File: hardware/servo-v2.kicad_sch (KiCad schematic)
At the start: 44 parts

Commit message: fix symbols
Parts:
- C1, C12: value (none) -> 10uF; footprint (none) -> kicad-libraries:C0805
- C10, C11: value (none) -> 100nF; footprint (none) -> kicad-libraries:C0603
- C2: value (none) -> 1uF; footprint (none) -> kicad-libraries:C0603F
- C3, C4, C5: value (none) -> 100nF; footprint (none) -> kicad-libraries:C0603F
- C6: value (none) -> 220nF; footprint (none) -> kicad-libraries:C0603F
- C7: value (none) -> 220pF; footprint (none) -> kicad-libraries:C0402F
- C8, C9: value (none) -> 10pF; footprint (none) -> kicad-libraries:C0603F
- D1: value (none) -> Z12V; footprint (none) -> kicad-libraries:SOD-123
- D3: value (none) -> blue; footprint (none) -> kicad-libraries:D0603E
- P1: value (none) -> CON-SENSOR2; footprint (none) -> kicad-libraries:CON-SENSOR2
- P2: value (none) -> BOOT; footprint (none) -> kicad-libraries:SolderJumper
- P3: value (none) -> DEBUG; footprint (none) -> kicad-libraries:DEBUG_PAD
- P4: value (none) -> black; footprint (none) -> kicad-libraries:OQ_2P
- Q1: value (none) -> FDS8449; footprint (none) -> kicad-libraries:SOIC-8-MOSFET
- R1, R3: value (none) -> 1k; footprint (none) -> kicad-libraries:R0603F
- R10, R11, R12, R13, R4, R5, R6, R7, R8, R9: value (none) -> 0R1; footprint (none) -> kicad-libraries:R0805E
- R16: value (none) -> 100k; footprint (none) -> kicad-libraries:R0603F
- R2: value (none) -> 10k; footprint (none) -> kicad-libraries:R0603F
- RP1: value (none) -> 82; footprint (none) -> kicad-libraries:4X0402
- U1: value (none) -> XMC1404; footprint (none) -> kicad-libraries:QFN48-EP2
- U2, U3, U4, U5: value (none) -> DRILL; footprint (none) -> kicad-libraries:DRILL_NP
- U6, U7: value (none) -> 74HC245; footprint (none) -> kicad-libraries:TSSOP20
- U8, U9: value (none) -> Con_Servo_5x; footprint (none) -> kicad-libraries:pin_array_5x3
- X1: value (none) -> 16MHz; footprint (none) -> kicad-libraries:CRYSTAL_3225
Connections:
- net CUR-SERVO-0: now also R8.1, U1.8 (P2.5_AI), U8.A1 (-)
- net CUR-SERVO-1: now also R7.1, U1.9 (P2.6_AI), U8.B1 (-)
- net CUR-SERVO-2: now also R6.1, U1.10 (P2.7_AI), U8.C1 (-)
- net CUR-SERVO-3: now also R5.1, U1.11 (P2.8_AI), U8.D1 (-)
- net CUR-SERVO-4: now also R4.1, U1.12 (P2.9_AI), U8.E1 (-)
- net CUR-SERVO-5: now also R13.1, U1.3 (P2.0_AIO), U9.A1 (-)
- net CUR-SERVO-6: now also R12.1, U1.4 (P2.1_AIO), U9.B1 (-)
- net CUR-SERVO-7: now also R11.1, U1.5 (P2.2_AI), U9.C1 (-)
- net CUR-SERVO-8: now also R10.1, U1.6 (P2.3_AI), U9.D1 (-)
- net CUR-SERVO-9: now also R9.1, U1.7 (P2.4_AI), U9.E1 (-)
- net PWM-SERVO-0: now also U1.30 (P0.1_IO), U6.6 (A4)
- net PWM-SERVO-1: now also U1.32 (P0.3_IO), U6.5 (A3)
- net PWM-SERVO-2: now also U1.31 (P0.2_IO), U6.4 (A2)
- net PWM-SERVO-3: now also U1.29 (P0.0_IO), U6.3 (A1)
- net PWM-SERVO-4: now also U1.35 (P0.6_IO), U6.2 (A0)
- net PWM-SERVO-5: now also U1.43 (P0.12_IO), U7.6 (A4)
- net PWM-SERVO-6: now also U1.46 (P0.15_IO), U7.5 (A3)
- net PWM-SERVO-7: now also U1.40 (P0.9_IO/RTC_XTAL2), U7.4 (A2)
- net PWM-SERVO-8: now also U1.39 (P0.8_IO/RTC_XTAL1), U7.3 (A1)
- net PWM-SERVO-9: now also U1.36 (P0.7_IO), U7.2 (A0)
- net S-CLK: now also RP1.7 (R2), U1.23 (P1.3_IHO)
- net S-CS: now also RP1.8 (R1), U1.25 (P1.1_IHO)
- net S-MISO: now also RP1.5 (R4), U1.20 (P1.6_IHO)
- net S-MOSI: now also RP1.6 (R3), U1.24 (P1.2_IHO)
- net V-EXT: now also R2.2, R3.1, U1.13 (P2.10/AIO)
- new net: P1.4, RP1.1 (P1)
- new net: P1.5, RP1.2 (P2)
- new net: P1.6, RP1.3 (P3)
- new net: C7.1, P1.7, RP1.4 (P4)
- new net: C8.1, U1.41 (P0.10_IO/XTAL1)
- new net: C9.1, U1.42 (P0.11_IO/XTAL2)
- new net: R1.1, U1.1 (P4.6_IO)
- new net: P3.1 (P1), U1.47 (P4.4_IO)
- new net: P2.2 (P2), U1.48 (P4.5_IO)
- new net: D3.2 (K), R1.2
- new net: P4.1 (P1), U8.A2 (+), U8.B2 (+), U8.C2 (+), U8.D2 (+), U8.E2 (+), U9.A2 (+), U9.B2 (+), U9.C2 (+), U9.D2 (+), U9.E2 (+)
- new net: P4.2 (P2), Q1.D
- new net: D1.2 (K), Q1.G, R16.1
- new net: U7.14 (B4), U9.A3 (PWM)
- new net: U7.15 (B3), U9.B3 (PWM)
- new net: U7.16 (B2), U9.C3 (PWM)
- new net: U7.17 (B1), U9.D3 (PWM)
- new net: U7.18 (B0), U9.E3 (PWM)
- new net: U6.14 (B4), U8.A3 (PWM)
- new net: U6.15 (B3), U8.B3 (PWM)
- new net: U6.16 (B2), U8.C3 (PWM)
- new net: U6.17 (B1), U8.D3 (PWM)
- new net: U6.18 (B0), U8.E3 (PWM)
- new net +5V: C12.1, P1.1, U6.1 (DIR), U6.20 (VCC), U7.1 (DIR), U7.20 (VCC)
- new net GND: C1.1, C10.2, C11.1, C12.2, C2.1, C3.2, C4.2, C5.2, C6.2, C7.2, C8.2, C9.2, P1.2, P1.EP, P2.1 (P1), Q1.S, R10.2, R11.2, R12.2, R13.2, R3.2, R4.2, R5.2, R6.2, R7.2, R8.2, R9.2, U1.17 (VSS), U1.37 (VSSP), U1.EP (VSSP), U6.19 (nOE), U6.7 (A5), U7.19 (nOE), U7.7 (A5), X1.3
- new net VCC: C1.2, C2.2, C3.1, C4.1, C5.1, C6.1, D3.1 (A), P1.3, U1.18 (VDD), U1.19 (VDDP), U1.27 (VDDP), U1.38 (VDDP)

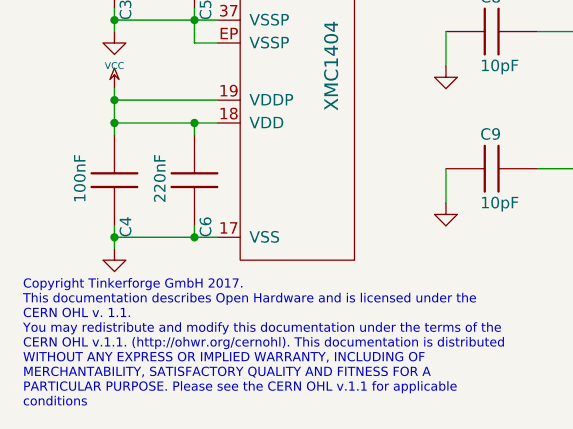
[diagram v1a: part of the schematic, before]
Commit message: Data Cleanup
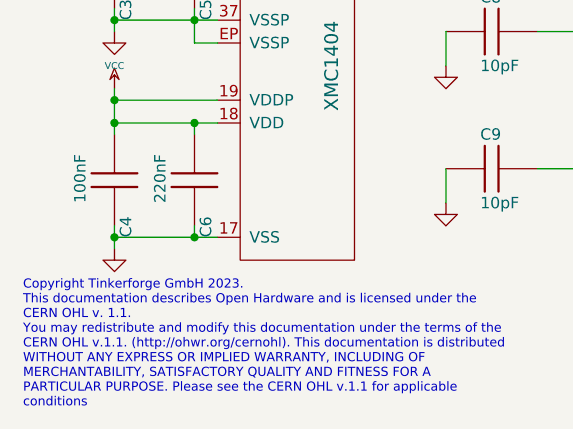
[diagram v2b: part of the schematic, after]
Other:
- note added: "Copyright Tinkerforge GmbH 2023. This documentation describes Open Hardware and is licensed under the CERN OHL v. 1.1. You may redistribute and modify this documentation under the terms of the CERN OHL v.1.1. (http://ohwr.org/cernohl). This documentation is distributed WITHOUT ANY EXPRESS OR IMPLIED WARRANTY, INCLUDING OF MERCHANTABILITY, SATISFACTORY QUALITY AND FITNESS FOR A PARTICULAR PURPOSE.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"
- note removed: "Copyright Tinkerforge GmbH 2017. This documentation describes Open Hardware and is licensed under the CERN OHL v. 1.1. You may redistribute and modify this documentation under the terms of the CERN OHL v.1.1. (http://ohwr.org/cernohl). This documentation is distributed WITHOUT ANY EXPRESS OR IMPLIED WARRANTY, INCLUDING OF MERCHANTABILITY, SATISFACTORY QUALITY AND FITNESS FOR A PARTICULAR PURPOSE.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"
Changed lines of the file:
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@@
   (title_block
     (title "Servo Bricklet")
-    (date "2019-06-17")
-    (rev "1.0")
+    (date "2023-01-25")
+    (rev "2.0")
     (company "Tinkerforge GmbH")
     (comment 1 "Licensed under CERN OHL v.1.1")
-    (comment 2 "Copyright (©) 2019, T.Schneidermann <tim@tinkerforge.com>")
+    (comment 2 "Copyright (©) 2023, T.Schneidermann <tim@tinkerforge.com>")
   )
   (junction (at 213.36 77.47) (diameter 0) (color 0 0 0 0)
@@
     (effects (font (size 0.9906 0.9906)) (justify left bottom))
   )
-  (text "Copyright Tinkerforge GmbH 2017.\nThis documentation describes Open Hardware and is licensed under the\nCERN OHL v. 1.1.\nYou may redistribute and modify this documentation under the terms of the\nCERN OHL v.1.1. (http://ohwr.org/cernohl). This documentation is distributed\nWITHOUT ANY EXPRESS OR IMPLIED WARRANTY, INCLUDING OF\nMERCHANTABILITY, SATISFACTORY QUALITY AND FITNESS FOR A\nPARTICULAR PURPOSE. Please see the CERN OHL v.1.1 for applicable\nconditions\n"
+  (text "Copyright Tinkerforge GmbH 2023.\nThis documentation describes Open Hardware and is licensed under the\nCERN OHL v. 1.1.\nYou may redistribute and modify this documentation under the terms of the\nCERN OHL v.1.1. (http://ohwr.org/cernohl). This documentation is distributed\nWITHOUT ANY EXPRESS OR IMPLIED WARRANTY, INCLUDING OF\nMERCHANTABILITY, SATISFACTORY QUALITY AND FITNESS FOR A\nPARTICULAR PURPOSE. Please see the CERN OHL v.1.1 for applicable\nconditions\n"
     (at 13.97 195.58 0)
     (effects (font (size 1.016 1.016)) (justify left bottom))
